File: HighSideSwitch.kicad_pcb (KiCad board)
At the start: 2 copper layers, 22 x 15.1 mm, 24 parts, among them J1 Conn_02x02, Q1 CSD18540Q5B, Q2 CSD18540Q5B, Q3 8050, U1 LM5060, U2 LM5050-1

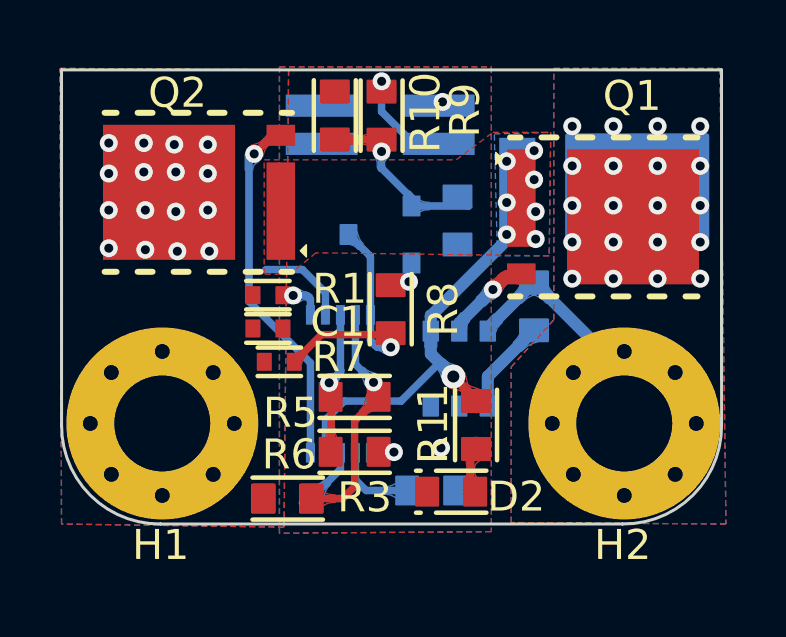
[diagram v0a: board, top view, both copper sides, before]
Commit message: iterative optimization
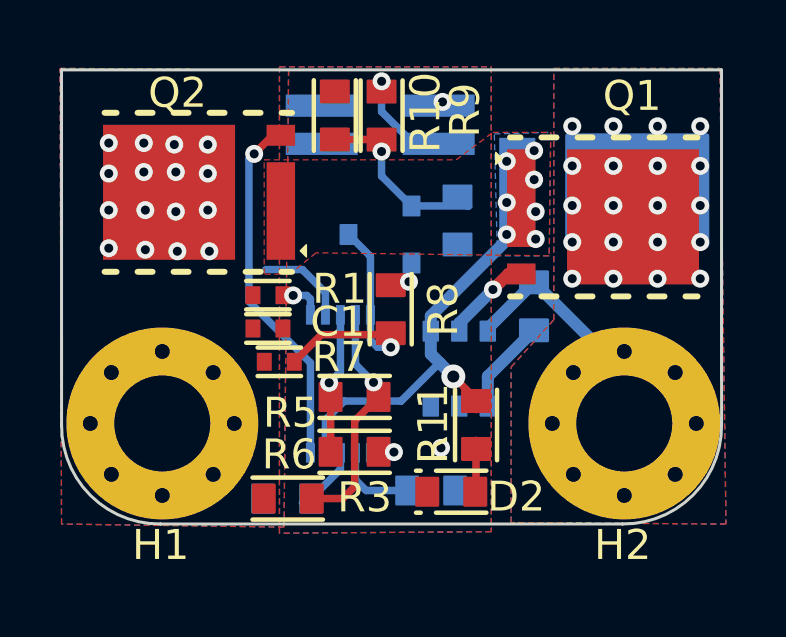
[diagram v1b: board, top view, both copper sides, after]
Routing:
- net /~{EN}: track 2.53 -> 3.36 mm
- net Net-(R5-Pad2): track 5.02 -> 4.49 mm
